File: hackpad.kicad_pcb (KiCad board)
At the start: 2 copper layers, 88.8 x 90 mm, 33 parts, among them SW1 RotaryEncoder_Switch, SW10 SW_Push, SW11 SW_Push, SW12 SW_Push, SW13 SW_Push, SW14 SW_Push, SW15 SW_Push, SW16 SW_Push, SW2 SW_Push, SW3 SW_Push, SW4 SW_Push, SW5 SW_Push, SW6 SW_Push, SW7 SW_Push, SW8 SW_Push, SW9 SW_Push, U1 MOUDLE-SEEEDUINO-XIAO

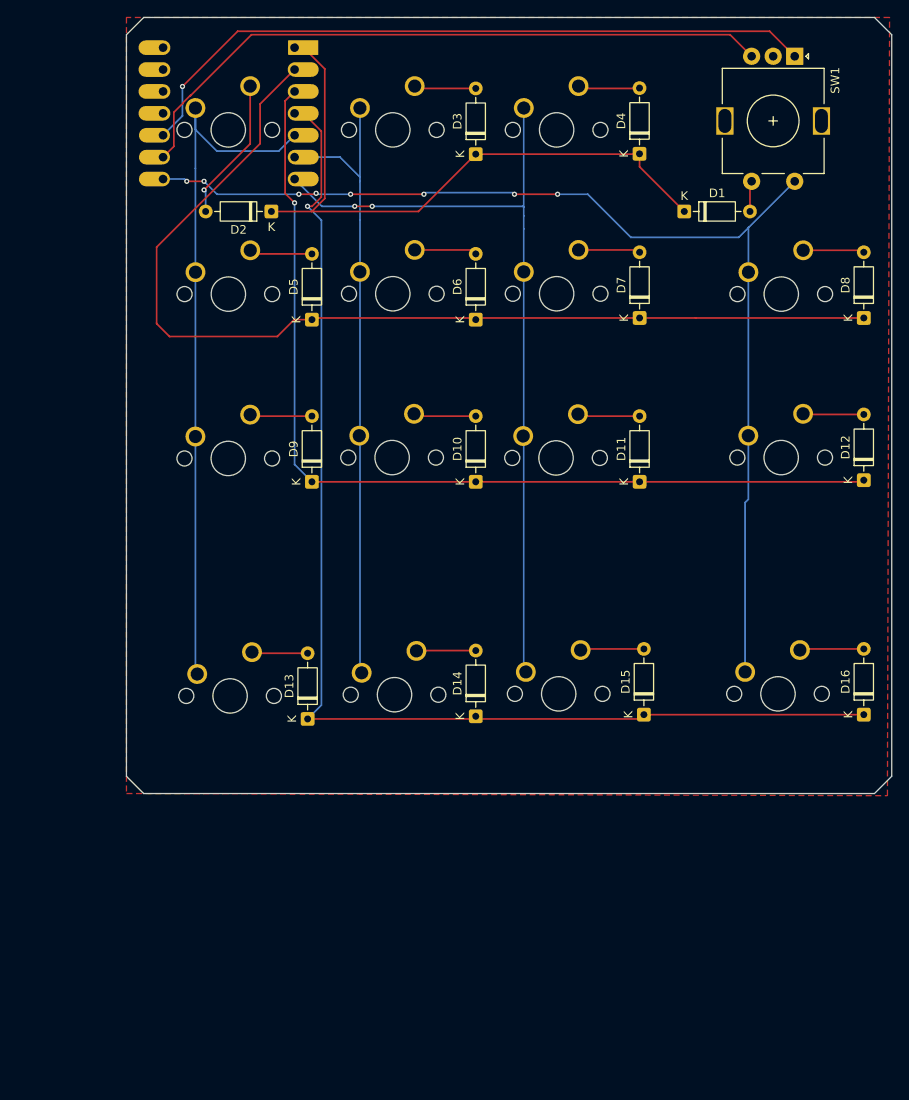
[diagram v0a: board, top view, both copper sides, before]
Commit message: I rediesinged it completly
Sorry for my horrible spelling
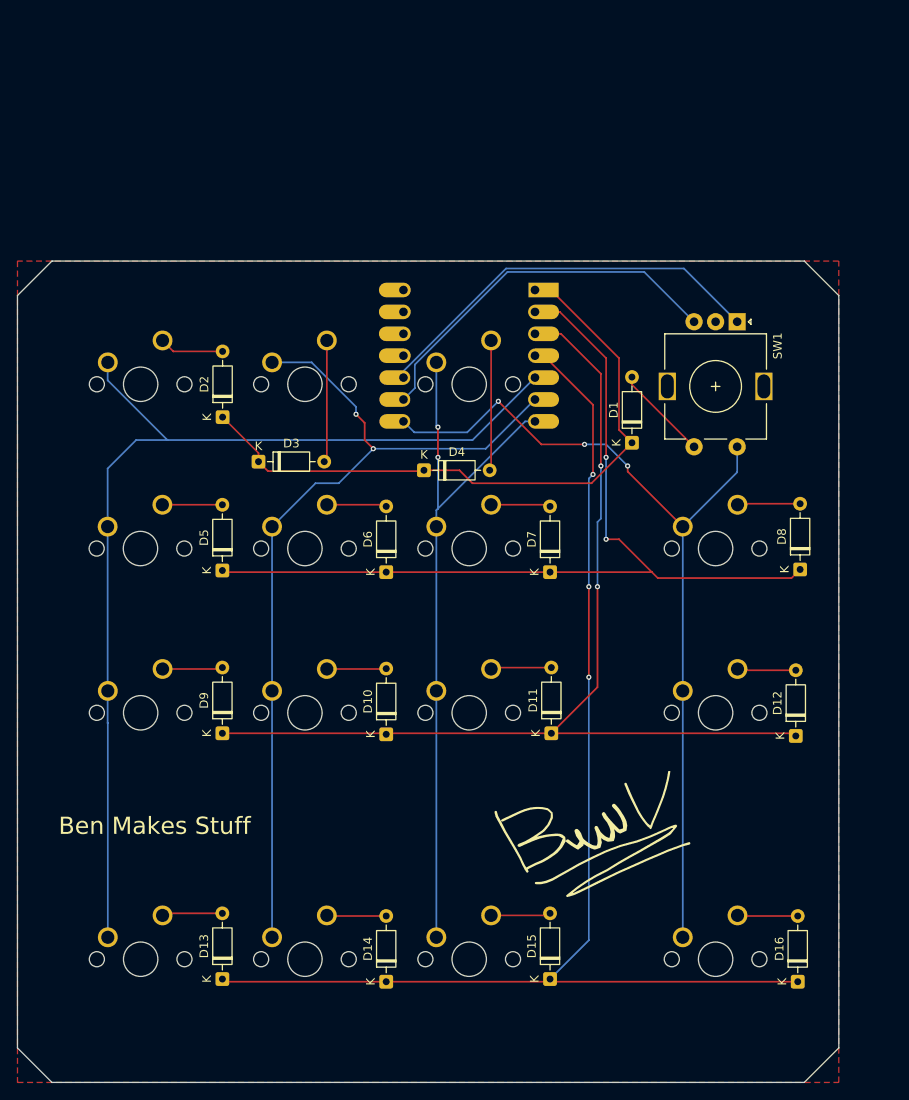
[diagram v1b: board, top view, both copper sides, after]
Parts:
- added  : LOGO, LOGO, F.Cu at (109.5, 161.9)
- added G***: LOGO, LOGO, F.Cu at (109.5, 161.9)
- moved D4 44.4 mm to (90.0, 119.5), turned to 0 degrees
- moved D3 43.7 mm to (70.8, 118.5), turned to 0 degrees
- moved U1 39.6 mm to (95.2, 106.2)
- moved D15 32.5 mm to (104.6, 178.5)
- moved D14 32.5 mm to (85.6, 178.8)
- moved SW15 32.5 mm to (95.2, 176.2)
- moved SW14 32.4 mm to (76.2, 176.2)
- moved SW13 32.2 mm to (57.1, 176.2)
- moved D16 31.9 mm to (133.3, 178.8)
- moved D13 31.7 mm to (66.6, 178.5)
- moved SW16 31.6 mm to (123.8, 176.2)
- moved SW1 31.5 mm to (126.3, 102.3)
- moved SW10 31.3 mm to (76.2, 147.6)
- moved SW6 31.3 mm to (76.2, 128.6)
- moved D7 31.2 mm to (104.6, 131.3)
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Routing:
- net /COL0: track 81.5 -> 120.2 mm, vias 0 -> 1
- net /POT1: track 81.4 -> 46.9 mm, vias 1 -> 0
- net /POT0: track 77.5 -> 43.8 mm
- net /COL3: track 130.7 -> 100.3 mm, vias 8 -> 3
- net /COL1: track 74.1 -> 101.8 mm, vias 0 -> 2
- net /ROW1: track 119.6 -> 106.6 mm, vias 0 -> 2
- net /COL2: track 93.5 -> 82.3 mm
- net Net-(D2-A): track 17.2 -> 7.51 mm, vias 1 -> 0
- net Net-(D4-A): track 7.19 -> 15.1 mm
- net /ROW2: track 112.8 -> 120.3 mm, vias 1 -> 2
- net Net-(D1-A): track 3.58 -> 11.1 mm
- net Net-(D3-A): track 7.19 -> 14.2 mm
- net /ROW3: track 139.1 -> 144.6 mm, vias 1 -> 3
- net /ROW0: track 75.9 -> 76.7 mm
- net Net-(D13-A): track 6.50 -> 7.03 mm
- added copper zone on F.Cu, net unconnected-(U1-GND-Pad13)
- removed copper zone on F.Cu, net /GND
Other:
- board size 88.8 x 90 mm -> 95.3 x 95.2 mm
- board text added: "Ben Makes Stuff"
